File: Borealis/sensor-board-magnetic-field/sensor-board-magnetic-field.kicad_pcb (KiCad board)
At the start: 2 copper layers, 35 x 30 mm, 4 parts, among them J2 Conn_01x03_Pin (data connecti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, J5 Conn_01x03_Pin (power connect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

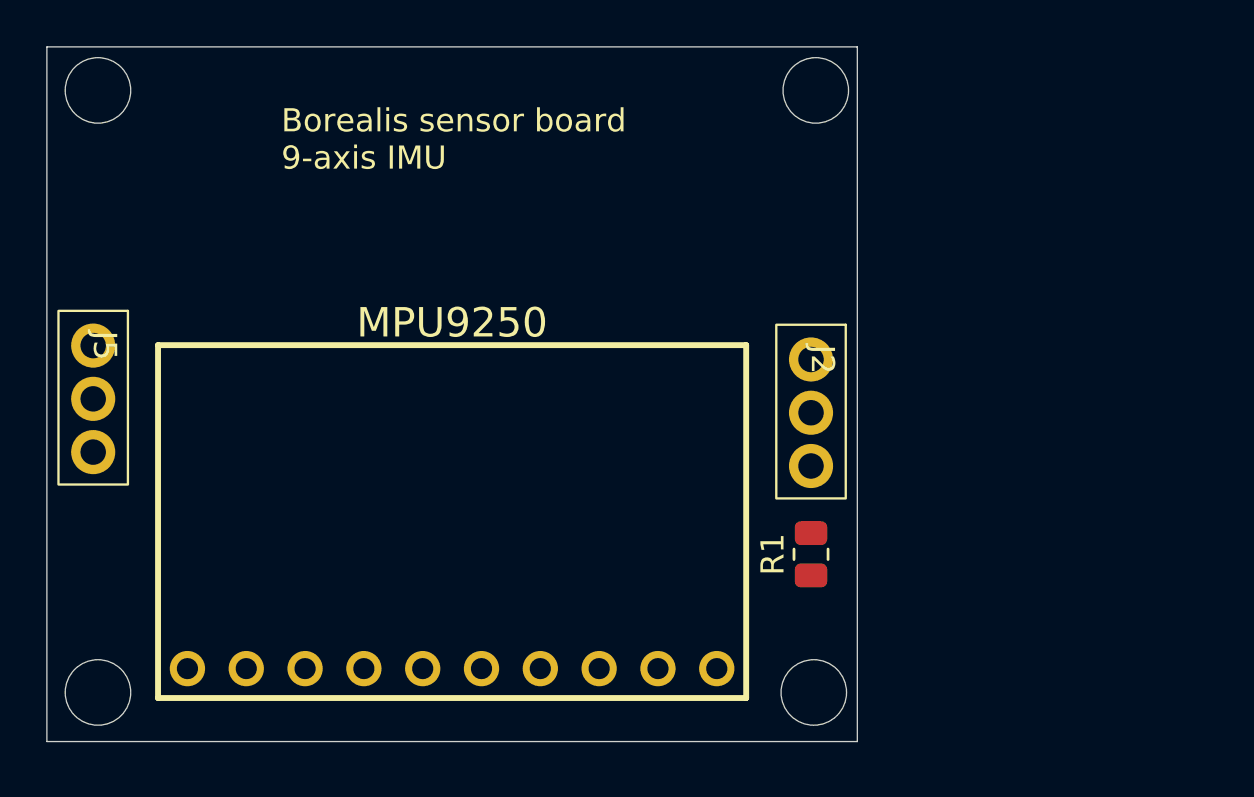
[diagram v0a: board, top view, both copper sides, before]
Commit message: updated
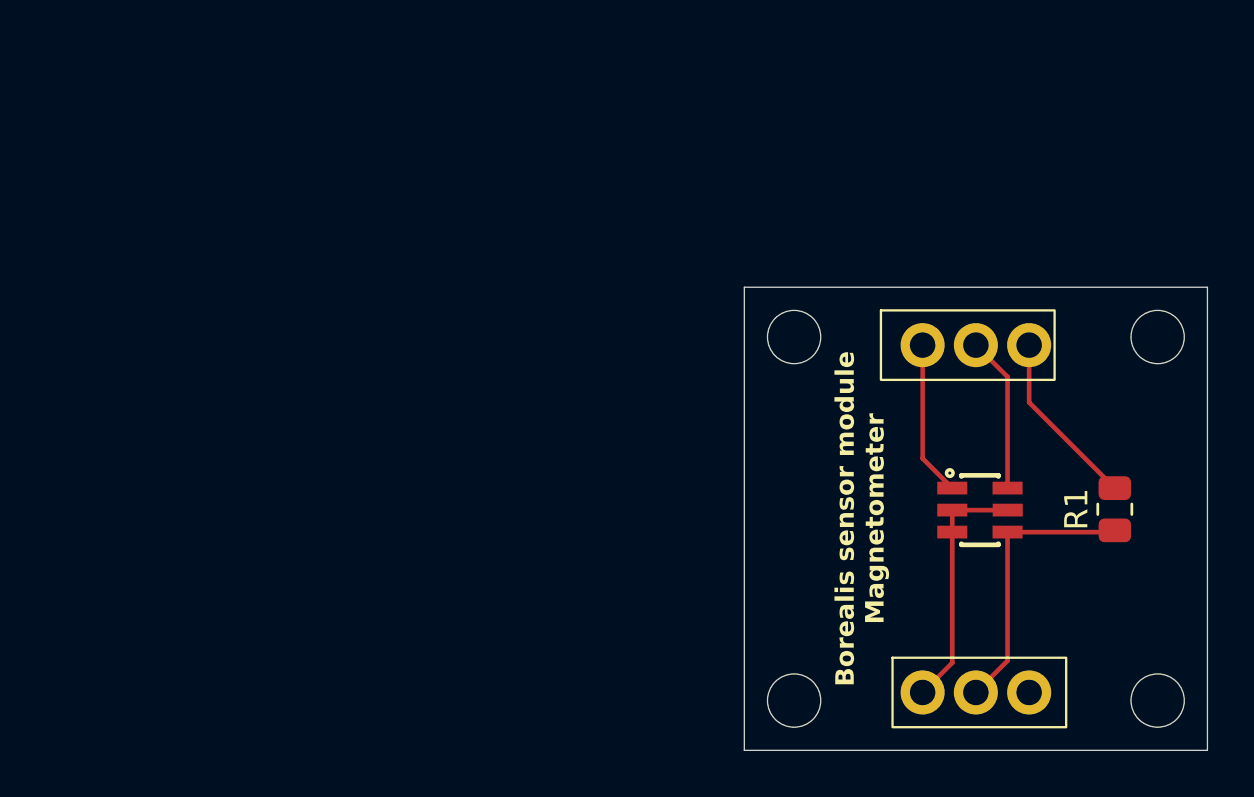
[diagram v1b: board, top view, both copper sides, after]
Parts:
- removed MPU9250: ~, batteryholder:MPU9250
- added TLV493D1: ~, batteryholder:TLV493D, F.Cu at (93.2, 118.1)
- moved J5 39.0 mm to (90.9, 126.0), turned to 0 degrees
- moved R1 13.3 mm to (99.0, 118.1)
- moved J2 4.56 mm to (90.4, 111.0), turned to 0 degrees
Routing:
- net +3.3V: track 0.00 -> 12.2 mm
- net GND: track 0.00 -> 10.8 mm
- net /ADC: track 0.00 -> 7.71 mm
- net /SDA: track 0.00 -> 6.74 mm
- net /SCL: track 0.00 -> 6.71 mm
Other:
- board size 35 x 30 mm -> 20 x 20 mm
- board text added: "Borealis sensor module Magnetometer"
- board text removed: "Borealis sensor board 9-axis IMU"
